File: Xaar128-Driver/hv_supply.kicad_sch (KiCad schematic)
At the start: 18 parts, among them Q7 DMG2305UX, Q8 DMG2305UX, U19 LTV-356T

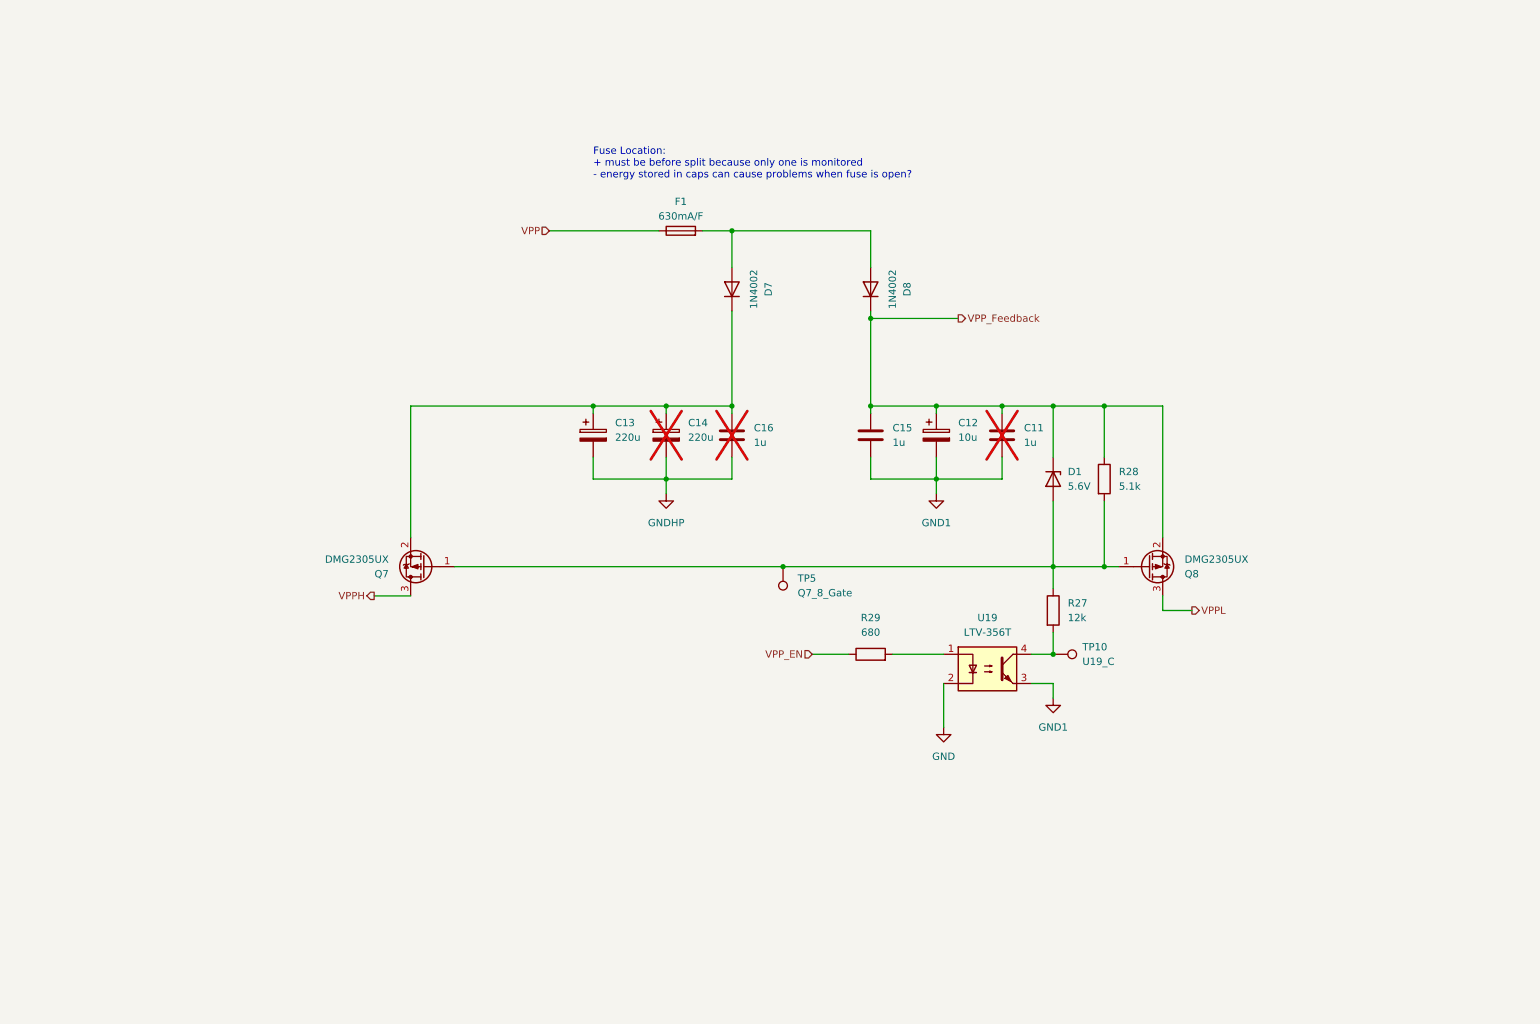
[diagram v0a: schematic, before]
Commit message: 5v monitoring
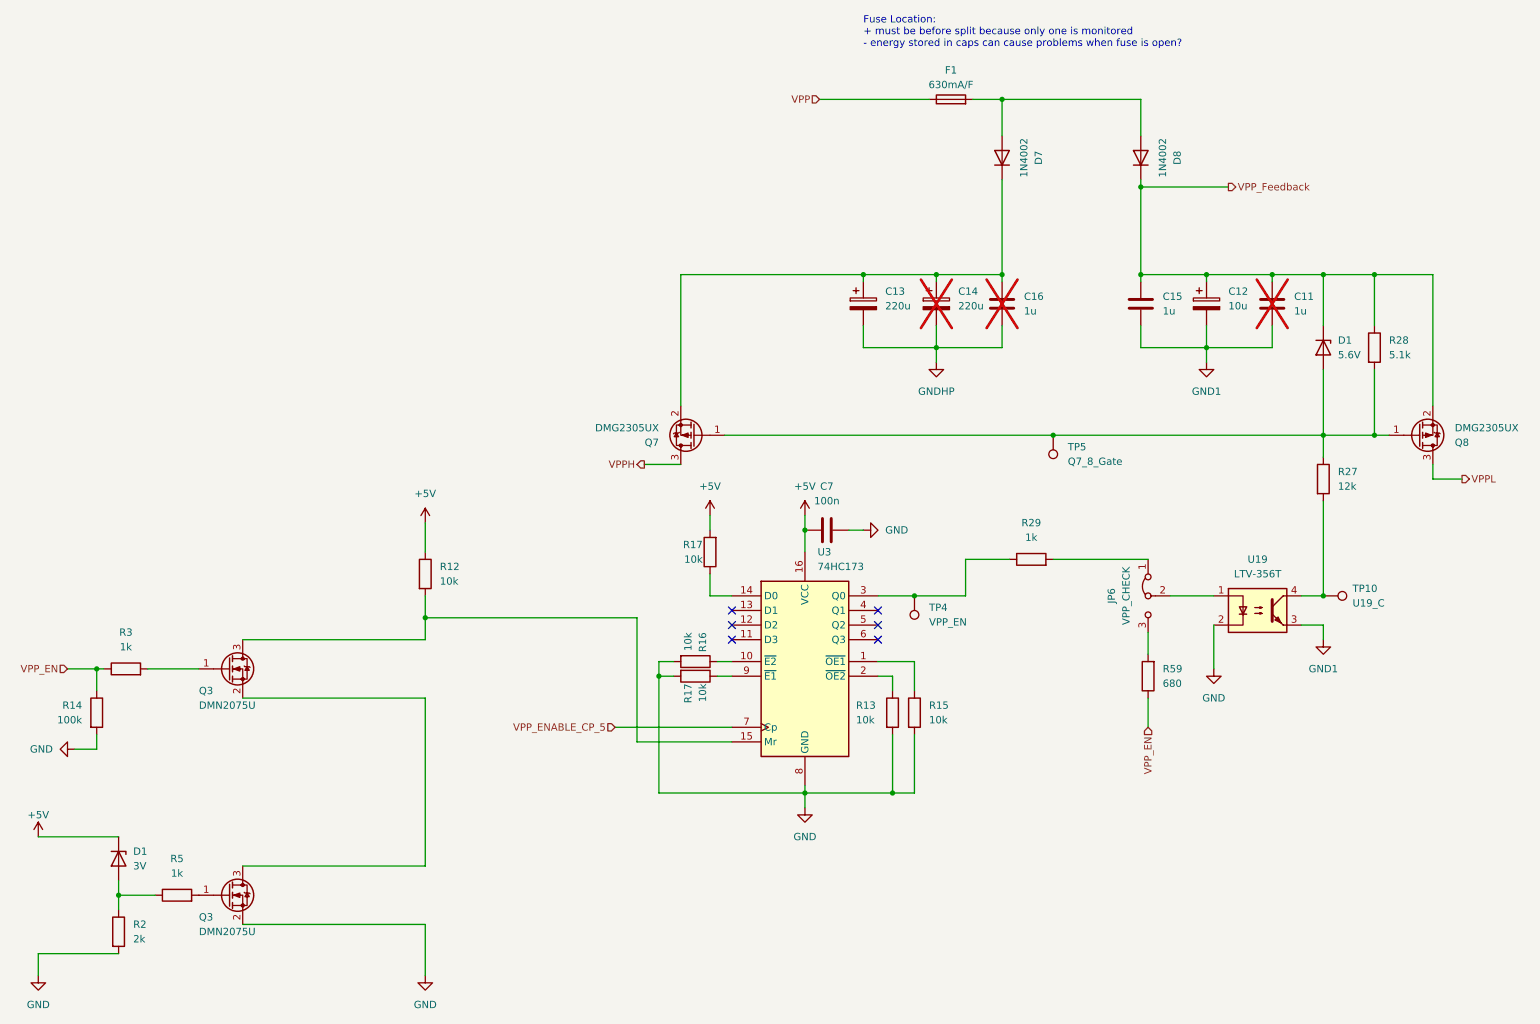
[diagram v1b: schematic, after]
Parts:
- added C7: 100n, symbol Device:C
- added D1: 3V, symbol Device:D_Zener
- added JP6: VPP_CHECK, symbol Jumper:Jumper_3_Bridged12
- added Q3 (x2): DMN2075U, Package_TO_SOT_SMD:SOT-23, symbol Transistor_FET:DMN2075U
- added R12, R13, R15, R16, R17 (x2): 10k, symbol Device:R
- added R14: 100k, symbol Device:R
- added R2: 2k, symbol Device:R
- added R3, R5: 1k, symbol Device:R
- added R59: 680, symbol Device:R
- added TP4: VPP_EN, symbol Connector:TestPoint
- added U3: 74HC173, symbol Xaar_Driver:74HC173
- R29: value 680 -> 1k
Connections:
- net GND: now also C7.2, Q3.2 (S), R13.2, R14.2, R15.2, R16.2, R17.2, R2.2, U3.8 (GND)
- net VPP_EN: now also R14.1, R3.1, R59.1; no longer R29.1
- net at R29.2: now also JP6.1 (A); no longer U19.1
- new net: R16.1, U3.10 (~{E2})
- new net: R17.1, U3.9 (~{E1})
- new net: R15.1, U3.1 (~{OE1})
- new net: R17.1, U3.14 (D0)
- new net: Q3.3 (D), R12.2, U3.15 (Mr)
- new net: R13.1, U3.2 (~{OE2})
- new net: R29.1, TP4.1, U3.3 (Q0)
- new net: Q3.1 (G), R3.2
- new net: Q3.2 (S), Q3.3 (D)
- new net: Q3.1 (G), R5.2
- new net: JP6.3 (B), R59.2
- new net: D1.2 (A), R2.1, R5.1
- new net: JP6.2 (C), U19.1
- new net +5V: C7.1, D1.1 (K), R12.1, R17.2, U3.16 (VCC)
- new net VPP_ENABLE_CP_5: U3.7 (Cp)
- no-connect marks 0 -> 6
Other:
- moved on the sheet: C11, C12, C13, C14, C15, C16, D1, D7, D8, F1, Q7, Q8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
